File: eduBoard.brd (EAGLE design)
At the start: 110 x 87.6 mm, 26 parts, among them CN1 LED-RGB2, CN2 LED-RGB1, CN3 LED-RGB3, CN4 PWM-13/16

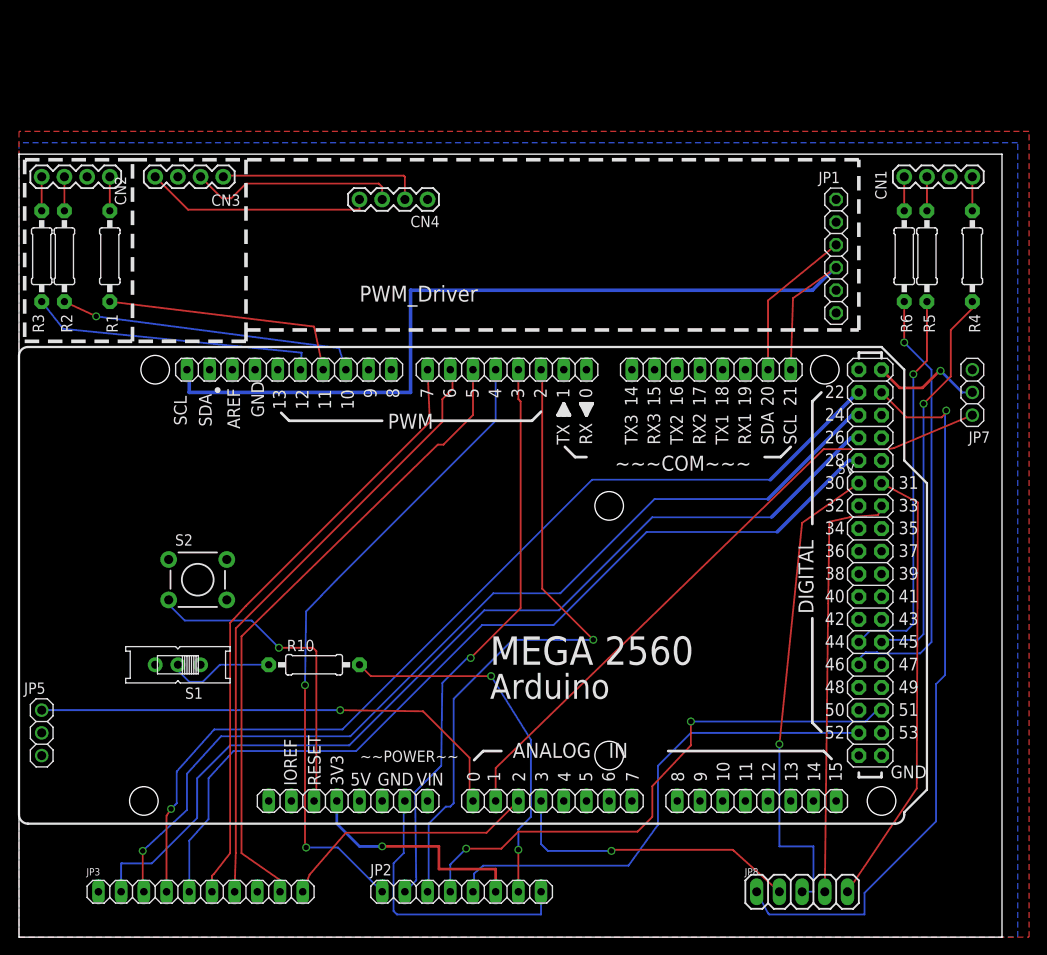
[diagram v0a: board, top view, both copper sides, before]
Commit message: routed
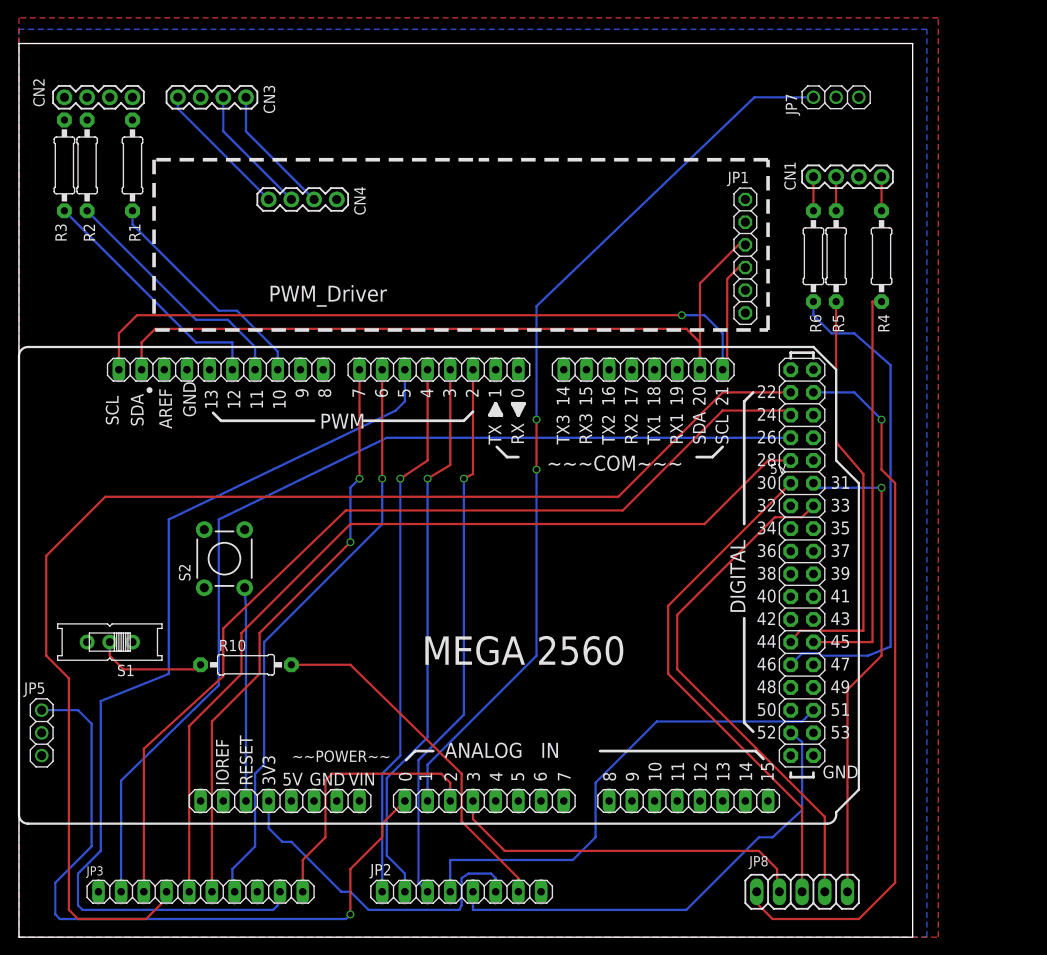
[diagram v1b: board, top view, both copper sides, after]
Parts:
- moved JP7 36.4 mm to (91.4, 94.0), turned to 0 degrees
- moved R1 10.5 mm to (12.7, 86.4)
- moved R2 10.5 mm to (7.62, 86.4)
- moved R3 10.5 mm to (5.08, 86.4)
- moved CN1 10.2 mm to (96.5, 85.1)
- moved R4 10.2 mm to (96.5, 76.2)
- moved CN4 10.2 mm to (35.6, 82.5)
- moved JP1 10.2 mm to (81.3, 76.2)
- moved R5 10.2 mm to (91.4, 76.2)
- moved R6 10.2 mm to (88.9, 76.2)
- moved CN2 9.25 mm to (12.7, 94.0)
- moved CN3 9.25 mm to (17.8, 94.0)
- moved S1 8.03 mm to (10.2, 33.0)
- moved R10 7.62 mm to (25.4, 30.5)
- moved XIO 7.62 mm to (87.6, 41.9)
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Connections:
- net PB4: now also R1.1; no longer R2.1
- net PB5: now also R2.1; no longer R1.1
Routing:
- net SDA: track 17.6 -> 86.4 mm
- net PA0: track 107.9 -> 144.8 mm, vias 1 -> 0
- net PE3: track 71.9 -> 107.0 mm
- net GND: track 32.1 -> 0.00 mm
- net ADC1: track 72.3 -> 101.3 mm, vias 0 -> 2
- net ADC0: track 55.0 -> 77.9 mm
- net +5V: track 12.8 -> 0.00 mm, vias 1 -> 0
- net PE4: track 74.1 -> 61.6 mm
- net RESET: track 36.1 -> 23.9 mm, vias 1 -> 0
- net PG5: track 72.8 -> 60.9 mm, vias 2 -> 1
- net +3V3: track 26.5 -> 37.5 mm, vias 1 -> 0
- net SCL: track 101.0 -> 90.3 mm, vias 0 -> 1
- net PC4: track 48.0 -> 58.1 mm
- net PWM16: track 25.5 -> 15.6 mm
- net PWM15: track 23.6 -> 14.6 mm
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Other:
- board size 110 x 87.6 mm -> 100 x 100 mm
- board text removed: "Arduino"
